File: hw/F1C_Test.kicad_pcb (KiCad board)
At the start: 2 copper layers, 66 parts, among them J1 USB_C_Receptacle_USB2.0_14P, J2 FPC/FFC P0.5, J3 1x03 P2.54, J4 1x06 P2.54, J5 AudioJack4, SW1 SW_Push, SW2 SW_Push, SW3 SW_SPST, U1 ME3103, U2 ME3103, U3 ME3103, U4 F1C100s, U5 W25Q32JVSS, U6 MT9284, Y1 24MHz 20pF

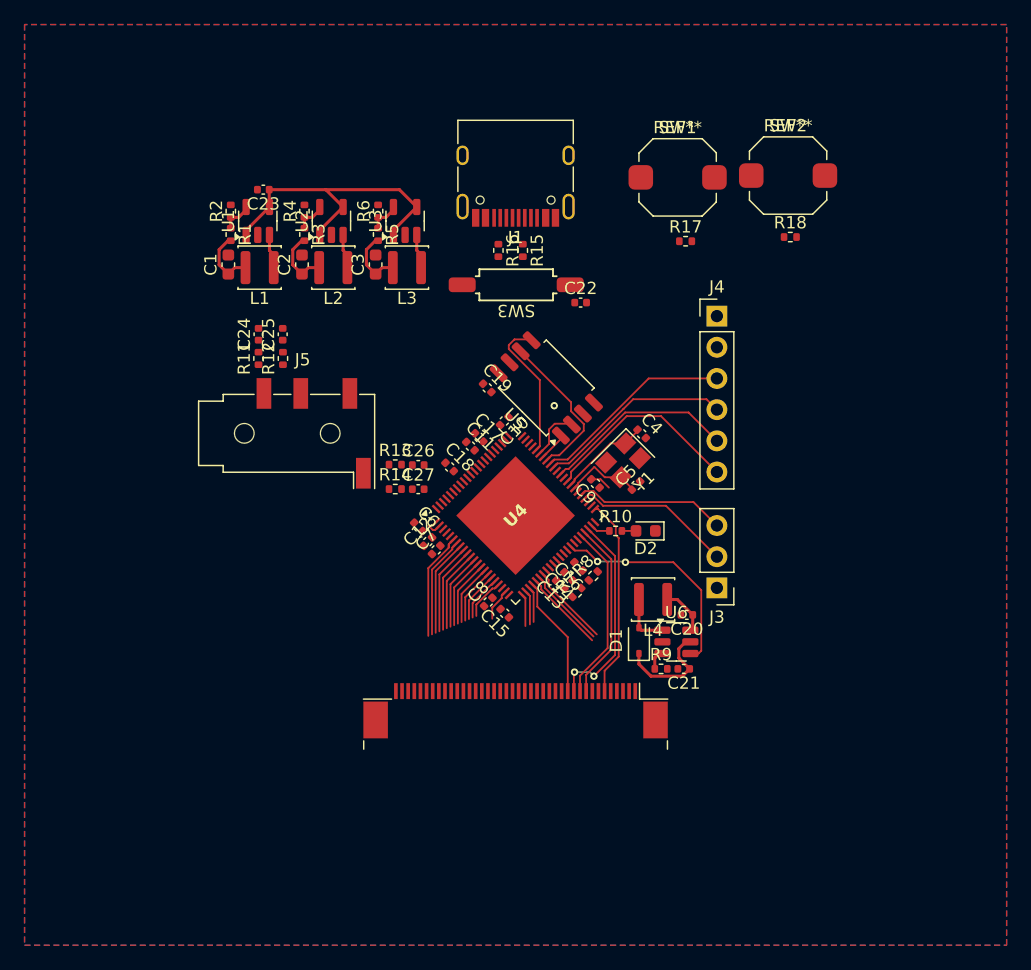
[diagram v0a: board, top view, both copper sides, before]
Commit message: hw: Layout & routing (WIP)
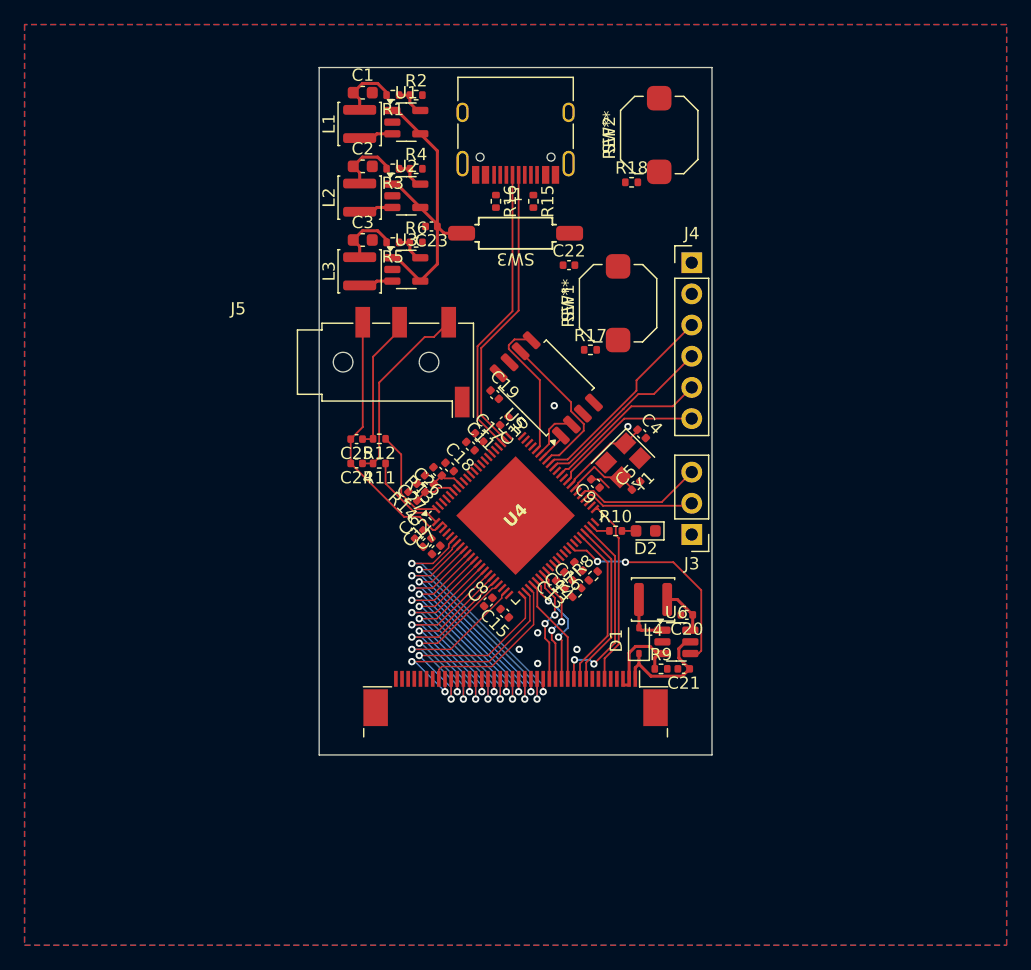
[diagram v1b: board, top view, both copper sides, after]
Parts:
- moved R2 17.8 mm to (131.9, 45.8), turned to 0 degrees
- moved C1 17.8 mm to (127.5, 45.5), turned to 0 degrees
- moved R1 17.4 mm to (130.0, 45.8), turned to 180 degrees
- moved U1 14.5 mm to (131.1, 48.0), turned to 0 degrees
- moved L1 14.3 mm to (127.3, 48.1), turned to 90 degrees
- moved C23 14.0 mm to (133.2, 56.5)
- moved R18 13.7 mm to (149.4, 52.9)
- moved C24 13.2 mm to (127.0, 75.8), turned to 180 degrees
- moved R11 13.0 mm to (128.9, 75.8), turned to 180 degrees
- moved R17 11.8 mm to (146.1, 66.5)
- moved SW1 11.3 mm to (148.3, 62.7), turned to 90 degrees
- moved SW2 11.0 mm to (151.7, 49.0), turned to 90 degrees
- moved C25 10.4 mm to (127.0, 73.8), turned to 180 degrees
- moved R12 10.2 mm to (128.9, 73.8), turned to 180 degrees
- moved J5 9.92 mm to (130.7, 67.5)
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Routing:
- net /USB_D+: track 0.00 -> 23.9 mm
- net /USB_D-: track 0.00 -> 23.7 mm
- net /HP_COM: track 1.21 -> 21.9 mm
- net /LCD_D21: track 2.64 -> 18.2 mm, vias 0 -> 2
- net /LCD_D22: track 2.83 -> 18.3 mm, vias 0 -> 2
- net Net-(C24-Pad1): track 0.00 -> 15.4 mm
- net /LCD_D20: track 2.66 -> 16.2 mm, vias 0 -> 2
- net /LCD_D18: track 3.76 -> 16.6 mm, vias 0 -> 2
- net /LCD_D19: track 3.42 -> 16.2 mm, vias 0 -> 2
- net /LCD_D15: track 4.14 -> 16.9 mm, vias 0 -> 2
- net /LCD_D14: track 4.56 -> 17.3 mm, vias 0 -> 2
- net /LCD_D13: track 4.97 -> 17.6 mm, vias 0 -> 2
- net /LCD_D12: track 5.39 -> 17.9 mm, vias 0 -> 2
- net /LCD_D11: track 5.80 -> 18.2 mm, vias 0 -> 2
- net /LCD_D10: track 6.22 -> 18.6 mm, vias 0 -> 2
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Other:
- board outline added: 32 x 56 mm
